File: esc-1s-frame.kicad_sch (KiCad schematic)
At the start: 21 parts, among them J1 Bat, J2 Conn_01x04_MountingPin, J4 Motor, J5 Conn_01x03_MountingPin, U1 EFM8BB51F2G-A-QFN20

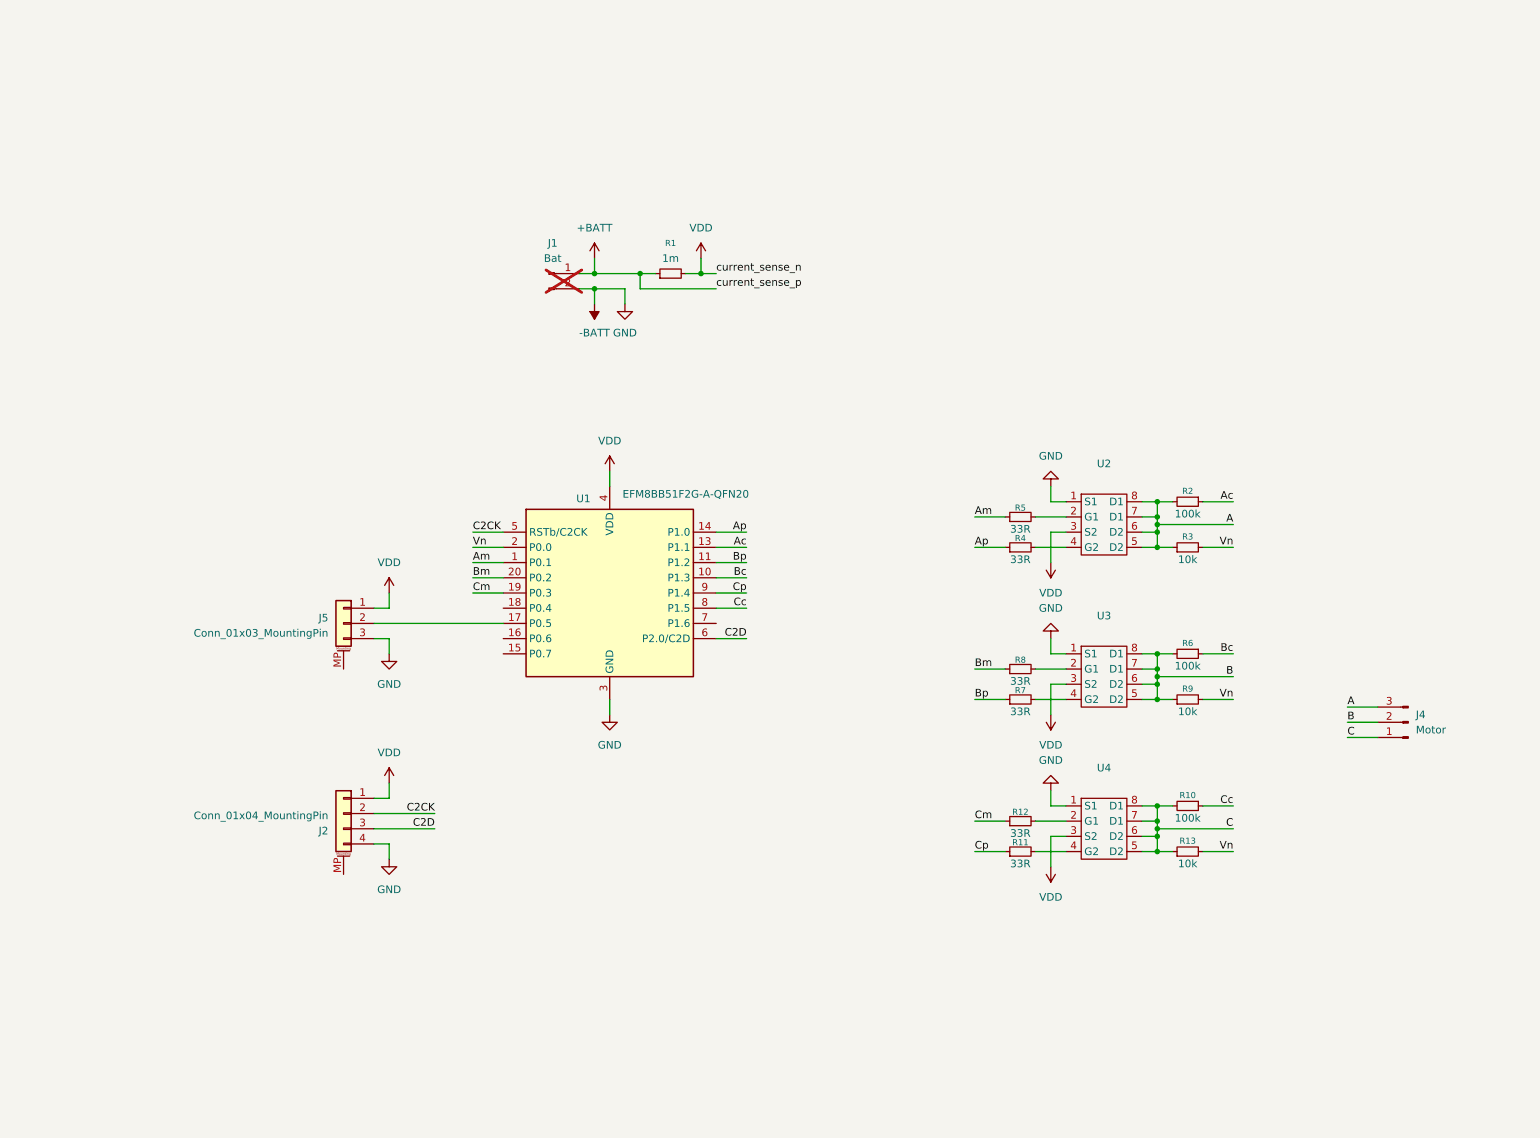
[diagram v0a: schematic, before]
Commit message: full board, sent to jlcpcb
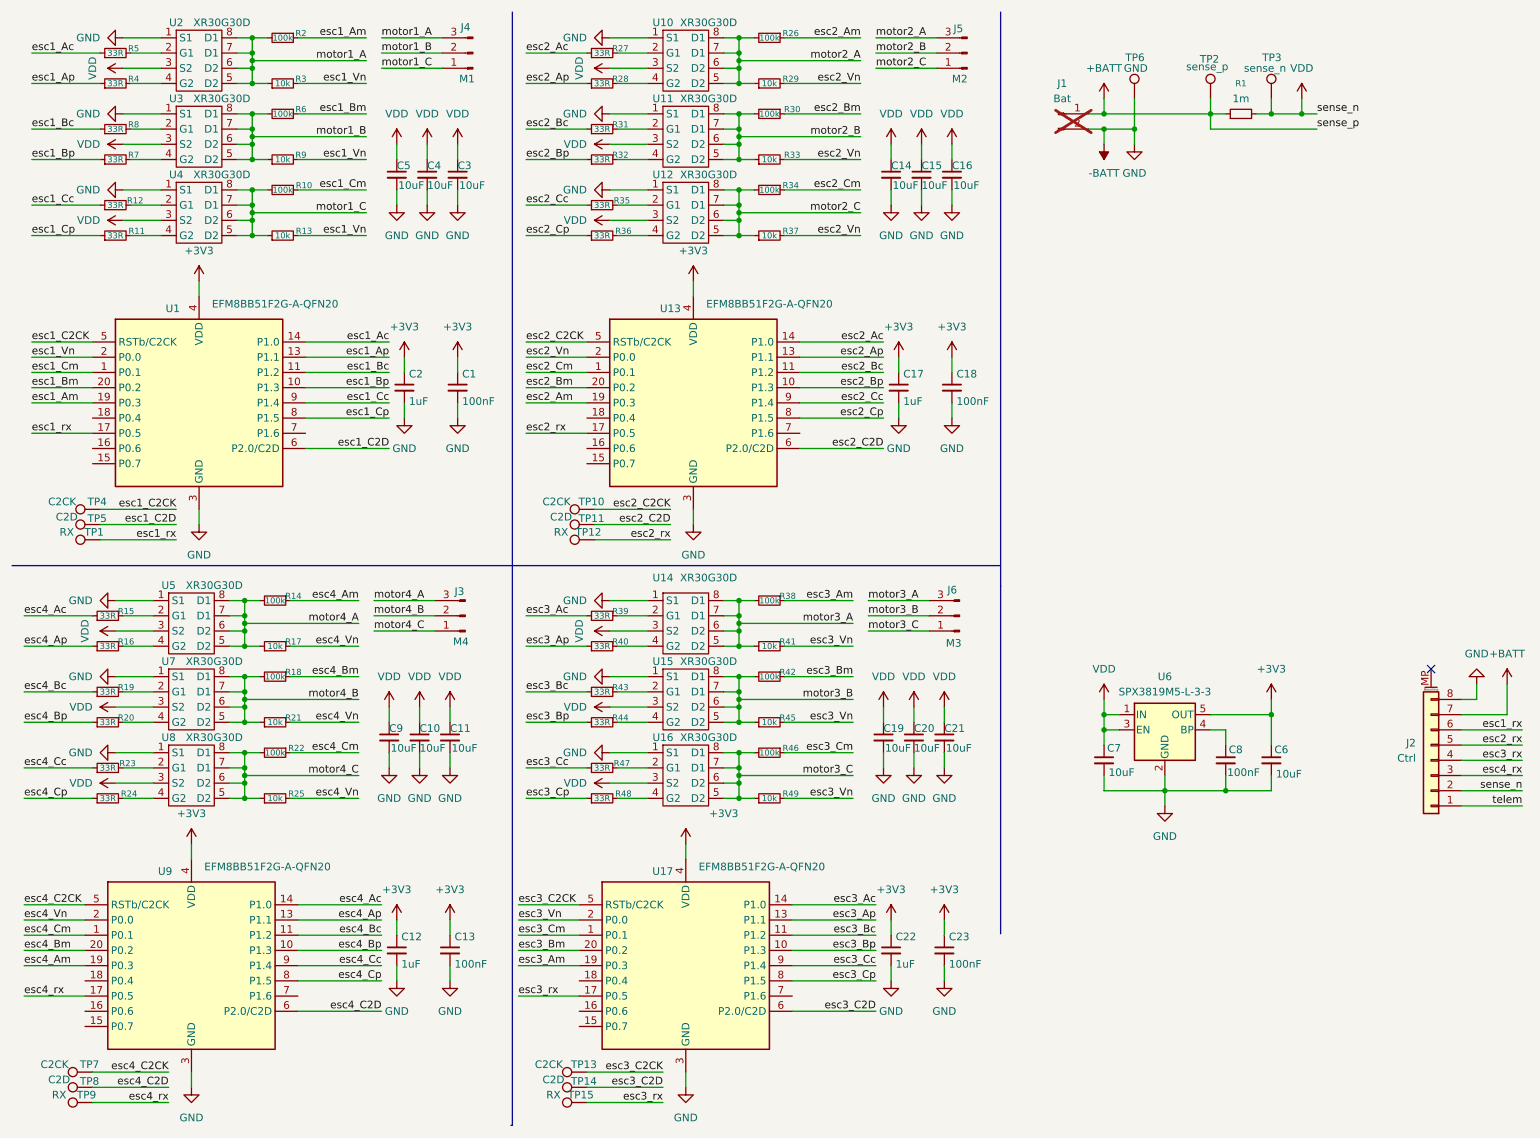
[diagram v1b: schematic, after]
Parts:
- removed J2: Conn_01x04_MountingPin, Connector_JST:JST_SH_SM04B-SRSS-TB_1x04-1MP_P1.00mm_Horizontal, symbol Connector_Generic_MountingPin:Conn_01x04_MountingPin
- removed J5: Conn_01x03_MountingPin, Connector_JST:JST_SH_SM03B-SRSS-TB_1x03-1MP_P1.00mm_Horizontal, symbol Connector_Generic_MountingPin:Conn_01x03_MountingPin
- added C1, C13, C18, C23, C8: 100nF, Capacitor_SMD:C_0402_1005Metric, symbol Device:C_Small
- added C10, C11, C14, C15, C16, C19, C20, C21, C3, C4, C5, C6, C7, C9: 10uF, Capacitor_SMD:C_0805_2012Metric, symbol Device:C_Small
- added C12, C17, C2, C22: 1uF, Capacitor_SMD:C_0402_1005Metric, symbol Device:C_Small
- added J2: Ctrl, Connector_JST:JST_SH_SM08B-SRSS-TB_1x08-1MP_P1.00mm_Horizontal, symbol Connector_Generic_MountingPin:Conn_01x08_MountingPin
- added J3: M4, Connector_Molex:Molex_PicoBlade_53048-0310_1x03_P1.25mm_Horizontal, symbol Connector:Conn_01x03_Pin
- added J5: M2, Connector_Molex:Molex_PicoBlade_53048-0310_1x03_P1.25mm_Horizontal, symbol Connector:Conn_01x03_Pin
- added J6: M3, Connector_Molex:Molex_PicoBlade_53048-0310_1x03_P1.25mm_Horizontal, symbol Connector:Conn_01x03_Pin
- added R14, R18, R22, R26, R30, R34, R38, R42, R46: 100k, Resistor_SMD:R_0402_1005Metric, symbol Device:R_Small
- added R15, R16, R19, R20, R23, R24, R27, R28, R31, R32, R35, R36, R39, R40, R43, R44, R47, R48: 33R, Resistor_SMD:R_0402_1005Metric, symbol Device:R_Small
- added R17, R21, R25, R29, R33, R37, R41, R45, R49: 10k, Resistor_SMD:R_0402_1005Metric, symbol Device:R_Small
- added TP1, TP12, TP15, TP9: RX, TestPoint:TestPoint_Pad_D1.0mm, symbol Connector:TestPoint
- added TP10, TP13, TP4, TP7: C2CK, TestPoint:TestPoint_Pad_D1.0mm, symbol Connector:TestPoint
- added TP11, TP14, TP5, TP8: C2D, TestPoint:TestPoint_Pad_D1.0mm, symbol Connector:TestPoint
- added TP2: sense_p, TestPoint:TestPoint_Pad_D1.0mm, symbol Connector:TestPoint
- added TP3: sense_n, TestPoint:TestPoint_Pad_D1.0mm, symbol Connector:TestPoint
- added TP6: GND, TestPoint:TestPoint_Pad_1.0x1.0mm, symbol Connector:TestPoint
- added U10, U11, U12, U14, U15, U16, U5, U7, U8: XR30G30D, Package_DFN_QFN:DFN-8-1EP_3x3mm_P0.65mm_EP1.55x2.4mm, symbol symbols:XR30G15D
- added U13, U17, U9: EFM8BB51F2G-A-QFN20, Package_DFN_QFN:SiliconLabs_QFN-20-1EP_3x3mm_P0.5mm_EP1.8x1.8mm, symbol MCU_SiliconLabs:EFM8BB10F2G-A-QFN20
- added U6: SPX3819M5-L-3-3, Package_TO_SOT_SMD:SOT-23-5, symbol Regulator_Linear:SPX3819M5-L-3-3
- J4: value Motor -> M1; footprint Connector_Molex:Molex_PicoBlade_53047-0310_1x03_P1.25mm_Vertical -> Connector_Molex:Molex_PicoBlade_53048-0310_1x03_P1.25mm_Horizontal
- U2, U3, U4: value ~ -> XR30G30D
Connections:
- net +BATT: now also J2.7 (Pin_7), TP2.1
- net -BATT: now also C1.2, C10.2, C11.2, C12.2, C13.2, C14.2, C15.2, C16.2, C17.2, C18.2, C19.2, C2.2, C20.2, C21.2, C22.2, C23.2, C3.2, C4.2, C5.2, C6.2, C7.2, C8.2, C9.2, J2.8 (Pin_8), TP6.1, U10.1 (S1), U11.1 (S1), U12.1 (S1), U13.12 (GND), U13.21 (GND), U13.3 (GND), U14.1 (S1), U15.1 (S1), U16.1 (S1), U17.12 (GND), U17.21 (GND), U17.3 (GND), U5.1 (S1), U6.2 (GND), U7.1 (S1), U8.1 (S1), U9.12 (GND), U9.21 (GND), U9.3 (GND)
- net VDD: now also C10.1, C11.1, C14.1, C15.1, C16.1, C19.1, C20.1, C21.1, C3.1, C4.1, C5.1, C7.1, C9.1, J2.2 (Pin_2), TP3.1, U10.3 (S2), U11.3 (S2), U12.3 (S2), U14.3 (S2), U15.3 (S2), U16.3 (S2), U5.3 (S2), U6.1 (IN), U6.3 (EN), U7.3 (S2), U8.3 (S2); no longer U1.4 (VDD)
- net esc1_rx: now reaches U1.17 (P0.5)
- net esc1_rx: now also J2.6 (Pin_6), TP1.1
- net A renamed motor1_A
- net Ac renamed esc1_Am
- net esc1_Am: now also U1.19 (P0.3); no longer U1.13 (P1.1)
- net Am renamed esc1_Ac
- net esc1_Ac: now also U1.14 (P1.0); no longer U1.1 (P0.1)
- net Ap renamed esc1_Ap
- net esc1_Ap: now also U1.13 (P1.1); no longer U1.14 (P1.0)
- net B renamed motor1_B
- net Bc renamed esc1_Bm
- net esc1_Bm: now also U1.20 (P0.2); no longer U1.10 (P1.3)
- net Bm renamed esc1_Bc
- net esc1_Bc: now also U1.11 (P1.2); no longer U1.20 (P0.2)
- net Bp renamed esc1_Bp
- net esc1_Bp: now also U1.10 (P1.3); no longer U1.11 (P1.2)
- net C renamed motor1_C
- net C2CK renamed esc1_C2CK
- net esc1_C2CK: now also TP4.1
- net C2D renamed esc1_C2D
- net esc1_C2D: now also TP5.1
- net Cc renamed esc1_Cm
- net esc1_Cm: now also U1.1 (P0.1); no longer U1.8 (P1.5)
- net Cm renamed esc1_Cc
- net esc1_Cc: now also U1.9 (P1.4); no longer U1.19 (P0.3)
- net Cp renamed esc1_Cp
- net esc1_Cp: now also U1.8 (P1.5); no longer U1.9 (P1.4)
- net Vn renamed esc1_Vn
- new net: C8.1, U6.4 (BP)
- new net: R23.2, U8.2 (G1)
- new net: R24.2, U8.4 (G2)
- new net: R15.2, U5.2 (G1)
- new net: R16.2, U5.4 (G2)
- new net: R31.2, U11.2 (G1)
- new net: R32.2, U11.4 (G2)
- new net: R20.2, U7.4 (G2)
- new net: R35.2, U12.2 (G1)
- new net: R47.2, U16.2 (G1)
- new net: R19.2, U7.2 (G1)
- new net: R48.2, U16.4 (G2)
- new net: R43.2, U15.2 (G1)
- new net: R36.2, U12.4 (G2)
- new net: R27.2, U10.2 (G1)
- new net: R39.2, U14.2 (G1)
- new net: R28.2, U10.4 (G2)
- new net: R40.2, U14.4 (G2)
- new net: R44.2, U15.4 (G2)
- new net +3V3: C1.1, C12.1, C13.1, C17.1, C18.1, C2.1, C22.1, C23.1, C6.1, U1.4 (VDD), U13.4 (VDD), U17.4 (VDD), U6.5 (OUT), U9.4 (VDD)
- new net esc2_Ac: R27.1, U13.14 (P1.0)
- new net esc2_Am: R26.1, U13.19 (P0.3)
- new net esc2_Ap: R28.1, U13.13 (P1.1)
- new net esc2_Bc: R31.1, U13.11 (P1.2)
- new net esc2_Bm: R30.1, U13.20 (P0.2)
- new net esc2_Bp: R32.1, U13.10 (P1.3)
- new net esc2_C2CK: TP10.1, U13.5 (RSTb/C2CK)
- new net esc2_C2D: TP11.1, U13.6 (P2.0/C2D)
- new net esc2_Cc: R35.1, U13.9 (P1.4)
- new net esc2_Cm: R34.1, U13.1 (P0.1)
- new net esc2_Cp: R36.1, U13.8 (P1.5)
- new net esc2_Vn: R29.2, R33.2, R37.2, U13.2 (P0.0)
- new net esc2_rx: J2.5 (Pin_5), TP12.1, U13.17 (P0.5)
- new net esc3_Ac: R39.1, U17.14 (P1.0)
- new net esc3_Am: R38.1, U17.19 (P0.3)
- new net esc3_Ap: R40.1, U17.13 (P1.1)
- new net esc3_Bc: R43.1, U17.11 (P1.2)
- new net esc3_Bm: R42.1, U17.20 (P0.2)
- new net esc3_Bp: R44.1, U17.10 (P1.3)
- new net esc3_C2CK: TP13.1, U17.5 (RSTb/C2CK)
- new net esc3_C2D: TP14.1, U17.6 (P2.0/C2D)
- new net esc3_Cc: R47.1, U17.9 (P1.4)
- new net esc3_Cm: R46.1, U17.1 (P0.1)
- new net esc3_Cp: R48.1, U17.8 (P1.5)
- new net esc3_Vn: R41.2, R45.2, R49.2, U17.2 (P0.0)
- new net esc3_rx: J2.4 (Pin_4), TP15.1, U17.17 (P0.5)
- new net esc4_Ac: R15.1, U9.14 (P1.0)
- new net esc4_Am: R14.1, U9.19 (P0.3)
- new net esc4_Ap: R16.1, U9.13 (P1.1)
- new net esc4_Bc: R19.1, U9.11 (P1.2)
- new net esc4_Bm: R18.1, U9.20 (P0.2)
- new net esc4_Bp: R20.1, U9.10 (P1.3)
- new net esc4_C2CK: TP7.1, U9.5 (RSTb/C2CK)
- new net esc4_C2D: TP8.1, U9.6 (P2.0/C2D)
- new net esc4_Cc: R23.1, U9.9 (P1.4)
- new net esc4_Cm: R22.1, U9.1 (P0.1)
- new net esc4_Cp: R24.1, U9.8 (P1.5)
- new net esc4_Vn: R17.2, R21.2, R25.2, U9.2 (P0.0)
- new net esc4_rx: J2.3 (Pin_3), TP9.1, U9.17 (P0.5)
- new net motor2_A: J5.3 (Pin_3), R26.2, R29.1, U10.5 (D2), U10.6 (D2), U10.7 (D1), U10.8 (D1)
- new net motor2_B: J5.2 (Pin_2), R30.2, R33.1, U11.5 (D2), U11.6 (D2), U11.7 (D1), U11.8 (D1)
- new net motor2_C: J5.1 (Pin_1), R34.2, R37.1, U12.5 (D2), U12.6 (D2), U12.7 (D1), U12.8 (D1)
- new net motor3_A: J6.3 (Pin_3), R38.2, R41.1, U14.5 (D2), U14.6 (D2), U14.7 (D1), U14.8 (D1)
- new net motor3_B: J6.2 (Pin_2), R42.2, R45.1, U15.5 (D2), U15.6 (D2), U15.7 (D1), U15.8 (D1)
- new net motor3_C: J6.1 (Pin_1), R46.2, R49.1, U16.5 (D2), U16.6 (D2), U16.7 (D1), U16.8 (D1)
- new net motor4_A: J3.3 (Pin_3), R14.2, R17.1, U5.5 (D2), U5.6 (D2), U5.7 (D1), U5.8 (D1)
- new net motor4_B: J3.2 (Pin_2), R18.2, R21.1, U7.5 (D2), U7.6 (D2), U7.7 (D1), U7.8 (D1)
- new net motor4_C: J3.1 (Pin_1), R22.2, R25.1, U8.5 (D2), U8.6 (D2), U8.7 (D1), U8.8 (D1)
- new net telem: J2.1 (Pin_1)
- no-connect marks 0 -> 1
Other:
- moved on the sheet: J1, J4, R1, R10, R11, R12, R13, R2, R3, R4, R5, R6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
